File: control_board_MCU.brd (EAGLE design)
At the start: 77.5 x 35.6 mm, 49 parts, among them U1 ATMEGA168, Y1 16MHZ

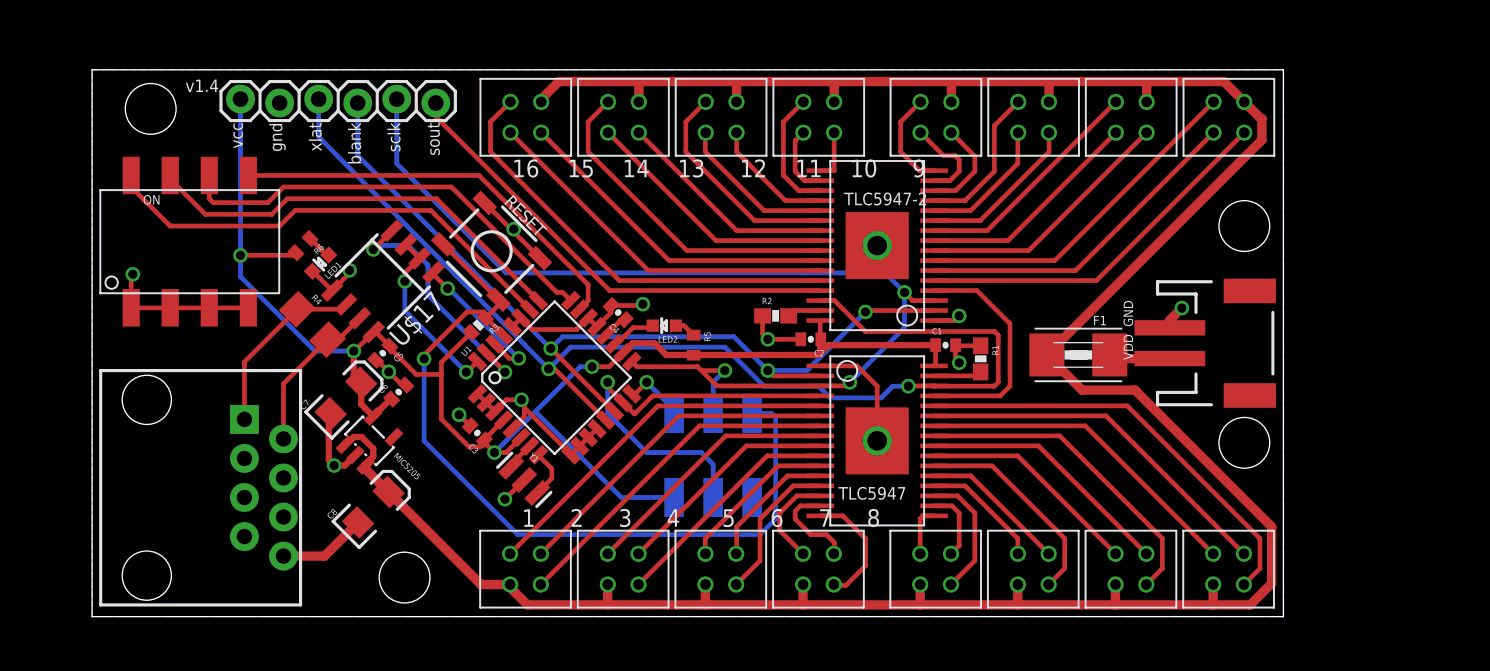
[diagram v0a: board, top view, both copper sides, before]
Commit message: new things!
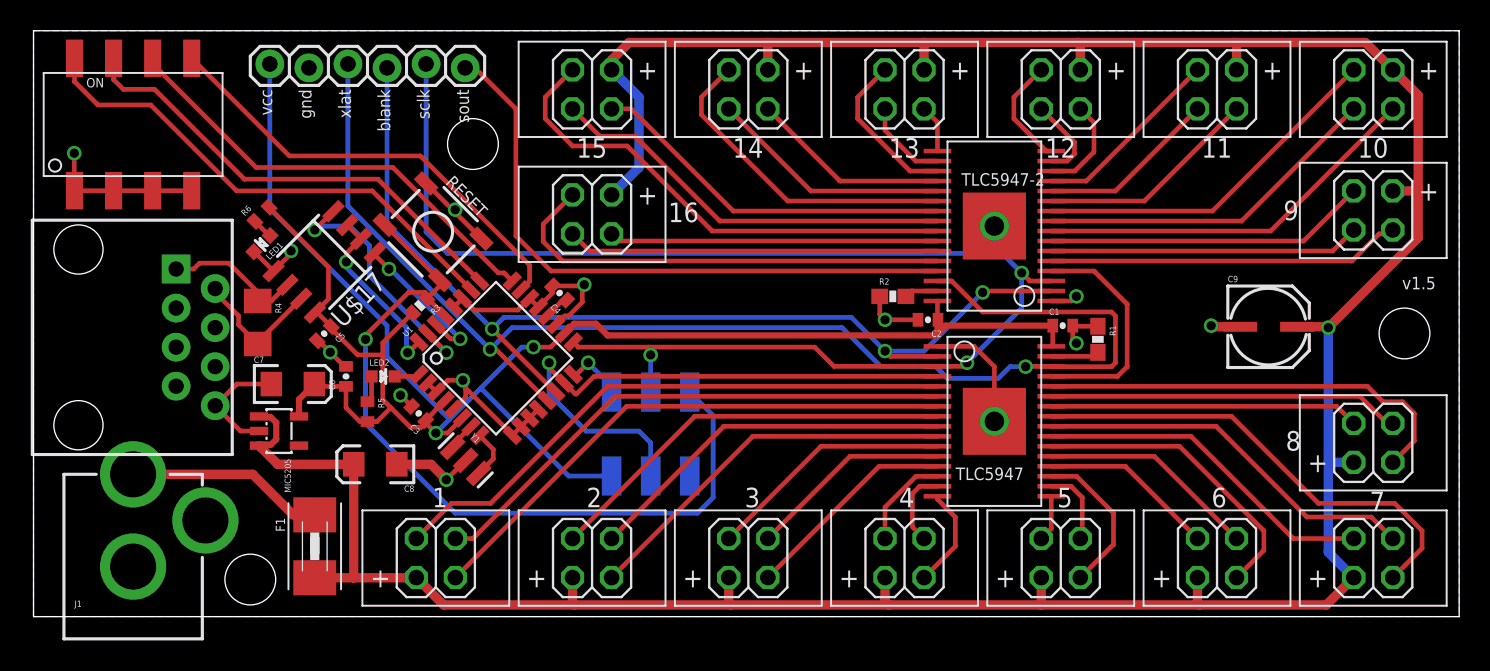
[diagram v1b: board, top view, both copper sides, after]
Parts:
- removed JP1: (no value), SparkFun-Connectors:JST-2-SMD
- removed STANDOFF3: STAND-OFF, SparkFun-Electromechanical:STAND-OFF
- removed U$1, U$10, U$11, U$12, U$13, U$14, U$15, U$16, U$2, U$3, U$4, U$5, U$6, U$7, U$8, U$9: SWR204-D02, SparkFun-Connectors:SWR204
- added 1, 10, 11, 12, 13, 14, 15, 16, 2, 3, 4, 5, 6, 7, 8, 9: (no value), pinhead:2X02
- added C9: 100uF, SparkFun-Capacitors:PANASONIC_C
- added J1: POWER_JACKPTH, SparkFun-Connectors:POWER_JACK_PTH
- moved F1 51.2 mm to (18.3, 4.57), turned to 270 degrees
- moved STANDOFF1 50.4 mm to (28.6, 30.7)
- moved STANDOFF2 31.3 mm to (14.1, 2.41)
- moved R5 21.6 mm to (21.7, 13.3)
- moved LED2 18.6 mm to (22.7, 15.6), turned to 270 degrees
- moved STANDOFF4 12.6 mm to (89.2, 18.4)
- moved U$18 10.7 mm to (2.92, 18.2)
- moved U$21 8.46 mm to (6.48, 32.0)
- moved C1 7.73 mm to (66.9, 18.9)
- moved R1 7.73 mm to (69.2, 18.0)
- moved R2 7.73 mm to (55.9, 20.8)
- moved TLC5947 7.73 mm to (62.5, 12.7)
- moved TLC5947-2 7.73 mm to (62.5, 25.4)
- moved C2 7.73 mm to (58.2, 19.3)
- moved MIC5205 5.91 mm to (16.0, 12.1), turned to 270 degrees
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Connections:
- removed net OUT1: TLC5947.6, U$1.P$2
- removed net OUT2: TLC5947.7, U$1.P$1
- new net N$14: 1.2, TLC5947.6
- new net N$9: 1.1, TLC5947.7
- net GND: now also C9.-, J1.GND, J1.GNDBREAK, U1.19; no longer JP1.1, U1.1
- net N$6: now also U1.1; no longer U1.19
- net N$8: now also J1.PWR; no longer JP1.2
- net OUT0: now also 1.3; no longer U$1.P$3
- net OUT10: now also 4.2; no longer U$4.P$2
- net OUT11: now also 4.1; no longer U$4.P$1
- net OUT12: now also 5.3; no longer U$5.P$3
- net OUT13: now also 5.2; no longer U$5.P$2
- net OUT14: now also 5.1; no longer U$5.P$1
- net OUT15: now also 6.3; no longer U$6.P$3
- net OUT16: now also 6.2; no longer U$6.P$2
- net OUT17: now also 6.1; no longer U$6.P$1
- net OUT18: now also 7.3; no longer U$7.P$3
- net OUT19: now also 7.2; no longer U$7.P$2
- net OUT20: now also 7.1; no longer U$7.P$1
- net OUT21: now also 8.3; no longer U$8.P$3
- net OUT22: now also 8.2; no longer U$8.P$2
- net OUT23: now also 8.1; no longer U$8.P$1
- net OUT24: now also 9.3; no longer U$9.P$3
- net OUT25: now also 9.2; no longer U$9.P$2
- net OUT26: now also 9.1; no longer U$9.P$1
- net OUT27: now also 10.3; no longer U$10.P$3
- net OUT28: now also 10.2; no longer U$10.P$2
- net OUT29: now also 10.1; no longer U$10.P$1
- net OUT3: now also 2.3; no longer U$3.P$3
- net OUT30: now also 11.3; no longer U$11.P$3
- net OUT31: now also 11.2; no longer U$11.P$2
- net OUT32: now also 11.1; no longer U$11.P$1
- net OUT33: now also 12.3; no longer U$12.P$3
- net OUT34: now also 12.2; no longer U$12.P$2
- net OUT35: now also 12.1; no longer U$12.P$1
- net OUT36: now also 13.3; no longer U$13.P$3
- net OUT37: now also 13.2; no longer U$13.P$2
- net OUT38: now also 13.1; no longer U$13.P$1
- net OUT39: now also 14.3; no longer U$14.P$3
- net OUT4: now also 2.2; no longer U$3.P$2
- net OUT40: now also 14.2; no longer U$14.P$2
- net OUT41: now also 14.1; no longer U$14.P$1
- net OUT42: now also 15.3; no longer U$15.P$3
- net OUT43: now also 15.2; no longer U$15.P$2
- net OUT44: now also 15.1; no longer U$15.P$1
- net OUT45: now also 16.3; no longer U$16.P$3
- net OUT46: now also 16.2; no longer U$16.P$2
- net OUT47: now also 16.1; no longer U$16.P$1
- net OUT5: now also 2.1; no longer U$3.P$1
- net OUT6: now also 3.3; no longer U$2.P$3
- net OUT7: now also 3.2; no longer U$2.P$2
- net OUT8: now also 3.1; no longer U$2.P$1
- net OUT9: now also 4.3; no longer U$4.P$3
- net VDD: now also 1.4, 10.4, 11.4, 12.4, 13.4, 14.4, 15.4, 16.4, 2.4, 3.4, 4.4, 5.4, 6.4, 7.4, 8.4, 9.4, C9.+; no longer U$1.P$4, U$10.P$4, U$11.P$4, U$12.P$4, U$13.P$4, U$14.P$4, U$15.P$4, U$16.P$4, U$2.P$4, U$3.P$4, U$4.P$4, U$5.P$4, U$6.P$4, U$7.P$4, U$8.P$4, U$9.P$4
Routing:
- net N$9: track 0.00 -> 36.0 mm
- net VCC: track 102.8 -> 138.5 mm, vias 4 -> 2
- net N$14: track 0.00 -> 35.2 mm
- net VDD: track 177.1 -> 207.7 mm, vias 0 -> 1
- net OUT2: track 22.4 -> 0.00 mm
- net OUT1: track 21.9 -> 0.00 mm
- net SCLK: track 69.7 -> 89.6 mm
- net OUT0: track 24.2 -> 38.0 mm
- net SIN: track 27.7 -> 38.9 mm
- net OUT44: track 21.5 -> 32.4 mm
- net SOUT1: track 30.6 -> 41.0 mm
- net XLAT: track 76.0 -> 86.1 mm
- net BLANK: track 58.3 -> 68.4 mm
- net OUT43: track 16.7 -> 26.8 mm
- net OUT3: track 17.0 -> 27.0 mm
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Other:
- board size 77.5 x 35.6 mm -> 92.7 x 38.1 mm
- board text added: "v1.5"
- board text removed: "1 2 3 4 5 6 7 8"
- board text removed: "16 15 14 13 12 11 10 9"
- board text removed: "VDD GND"
- board text removed: "v1.4"
